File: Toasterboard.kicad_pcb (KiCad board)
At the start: 2 copper layers, 2 parts, among them U1 LM341T-05_TO220, U2 NE555P

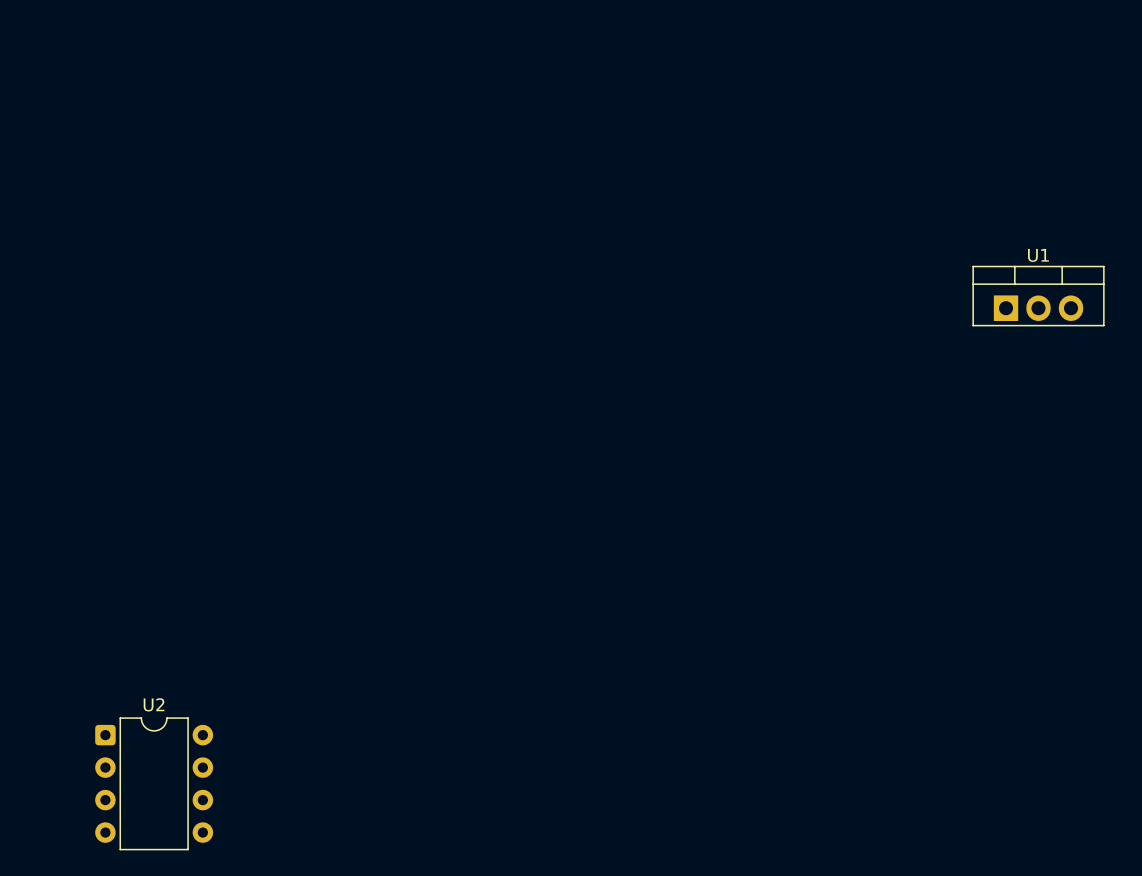
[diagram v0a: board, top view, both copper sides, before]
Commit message: feat: finished basic logics
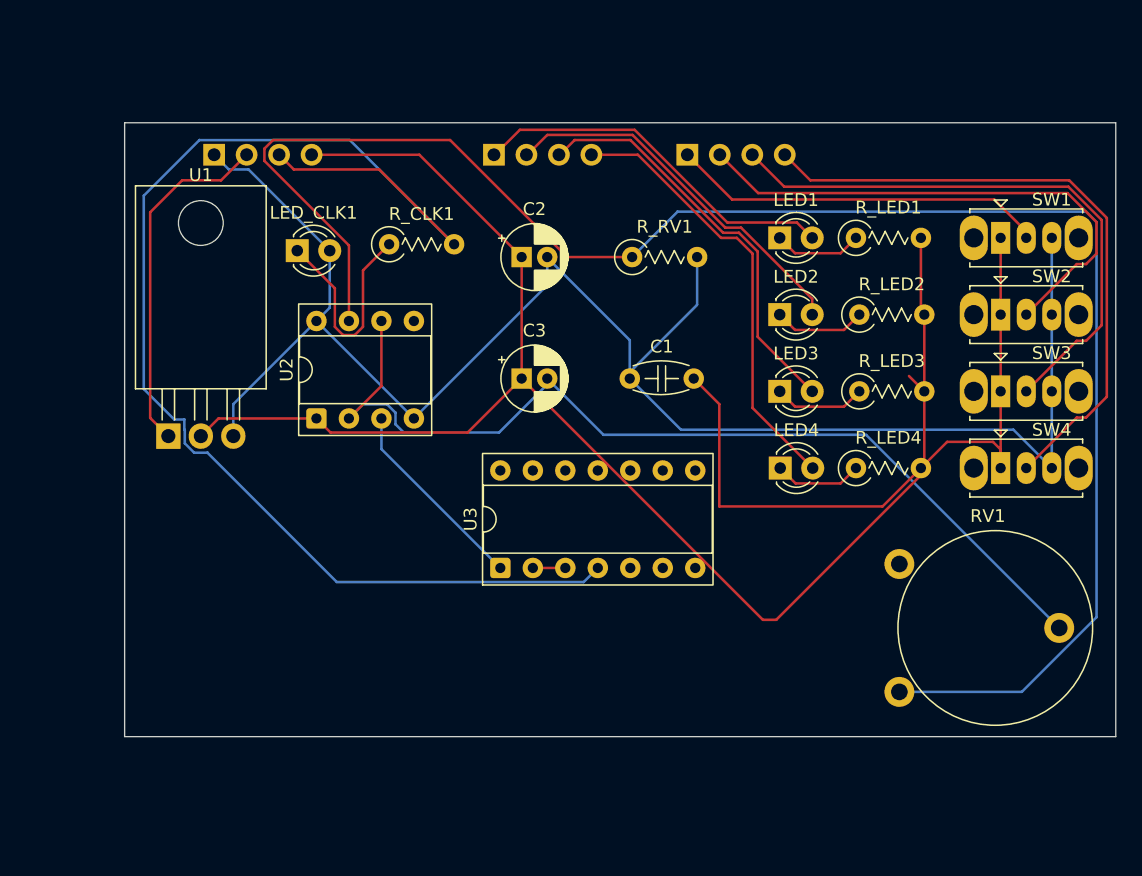
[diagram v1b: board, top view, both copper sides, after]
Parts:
- added C1: 0.01uF, PCM_Capacitor_THT_US_AKL:C_Disc_D5.0mm_W2.5mm_P5.00mm, F.Cu at (129.0, 88.5)
- added C2: 100uF, PCM_Capacitor_THT_US_AKL:CP_Radial_D5.0mm_P2.00mm, F.Cu at (120.5, 79.0)
- added C3: 100uF, PCM_Capacitor_THT_US_AKL:CP_Radial_D5.0mm_P2.00mm, F.Cu at (120.5, 88.5)
- added J1: Power, Connector_PinHeader_2.54mm:PinHeader_1x04_P2.54mm_Vertical, B.Cu at (96.5, 71.0)
- added J2: LEDs, Connector_PinHeader_2.54mm:PinHeader_1x04_P2.54mm_Vertical, B.Cu at (118.4, 71.0)
- added J3: Switches, Connector_PinHeader_2.54mm:PinHeader_1x04_P2.54mm_Vertical, B.Cu at (133.5, 71.0)
- added LED1: Red, LED_THT:LED_D3.0mm, F.Cu at (140.7, 77.5)
- added LED2: Red, LED_THT:LED_D3.0mm, F.Cu at (140.7, 83.5)
- added LED3: Red, LED_THT:LED_D3.0mm, F.Cu at (140.7, 89.5)
- added LED4: Red, LED_THT:LED_D3.0mm, F.Cu at (140.8, 95.5)
- added LED_CLK1: Green, LED_THT:LED_D3.0mm, F.Cu at (103.0, 78.5)
- added RV1: 10k, Potentiometer_THT:Potentiometer_Piher_PT-15-V02_Vertical, F.Cu at (150.1, 113.0)
- added R_CLK1: 1k, PCM_Resistor_THT_US_AKL:R_Axial_DIN0207_L6.3mm_D2.5mm_P5.08mm_Vertical, F.Cu at (110.2, 78.0)
- added R_LED1: 1k, PCM_Resistor_THT_US_AKL:R_Axial_DIN0207_L6.3mm_D2.5mm_P5.08mm_Vertical, F.Cu at (146.7, 77.5)
- added R_LED2: 1k, PCM_Resistor_THT_US_AKL:R_Axial_DIN0207_L6.3mm_D2.5mm_P5.08mm_Vertical, F.Cu at (146.9, 83.5)
- added R_LED3: 1k, PCM_Resistor_THT_US_AKL:R_Axial_DIN0207_L6.3mm_D2.5mm_P5.08mm_Vertical, F.Cu at (146.9, 89.5)
- added R_LED4: 1k, PCM_Resistor_THT_US_AKL:R_Axial_DIN0207_L6.3mm_D2.5mm_P5.08mm_Vertical, F.Cu at (146.7, 95.5)
- added R_RV1: 1k, PCM_Resistor_THT_US_AKL:R_Axial_DIN0207_L6.3mm_D2.5mm_P5.08mm_Vertical, F.Cu at (129.2, 79.0)
- added SW1: SW_SPDT, Button_Switch_THT:SW_Slide_SPDT_Straight_CK_OS102011MS2Q, F.Cu at (158.0, 77.5)
- added SW2: SW_SPDT, Button_Switch_THT:SW_Slide_SPDT_Straight_CK_OS102011MS2Q, F.Cu at (158.0, 83.5)
- added SW3: SW_SPDT, Button_Switch_THT:SW_Slide_SPDT_Straight_CK_OS102011MS2Q, F.Cu at (158.0, 89.5)
- added SW4: SW_SPDT, Button_Switch_THT:SW_Slide_SPDT_Straight_CK_OS102011MS2Q, F.Cu at (158.0, 95.5)
- added U3: 74LS14, Package_DIP:DIP-14_W7.62mm_Socket, F.Cu at (118.9, 103.3)
- U1: footprint Package_TO_SOT_THT:TO-220-3_Vertical -> Package_TO_SOT_THT:TO-220-3_Horizontal_TabDown
- U2: footprint Package_DIP:DIP-8_W7.62mm -> Package_DIP:DIP-8_W7.62mm_Socket
- moved U1 66.3 mm to (92.9, 93.0)
- moved U2 29.8 mm to (104.5, 91.6), turned to 90 degrees
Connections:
- U2 pad 2: unconnected-(U2-TRIG-Pad2) -> Net-(U2-THRES)
- U2 pad 4: unconnected-(U2-~{RST}-Pad4) -> +5V
- U2 pad 6: unconnected-(U2-THRES-Pad6) -> Net-(U2-THRES)
- U2 pad 7: unconnected-(U2-DISCH-Pad7) -> Net-(U2-DISCH)
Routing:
- net GND: track 0.00 -> 176.9 mm
- net Net-(U2-DISCH): track 0.00 -> 135.9 mm
- net +5V: track 0.00 -> 135.4 mm
- net /Clk: track 0.00 -> 104.4 mm
- net Net-(U2-THRES): track 0.00 -> 76.2 mm
- net Net-(J3-Pin_4): track 0.00 -> 49.8 mm
- net Net-(J3-Pin_3): track 0.00 -> 45.7 mm
- net Net-(J3-Pin_2): track 0.00 -> 41.6 mm
- net Net-(J2-Pin_4): track 0.00 -> 34.4 mm
- net Net-(J2-Pin_3): track 0.00 -> 32.2 mm
- net Net-(J3-Pin_1): track 0.00 -> 29.5 mm
- net Net-(J2-Pin_2): track 0.00 -> 29.5 mm
- net Net-(J2-Pin_1): track 0.00 -> 29.1 mm
- net +12V: track 0.00 -> 27.5 mm
- net Net-(LED_CLK1-K): track 0.00 -> 17.2 mm
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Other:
- board outline added: 77.5 x 48 mm

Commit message: feat: finish routing
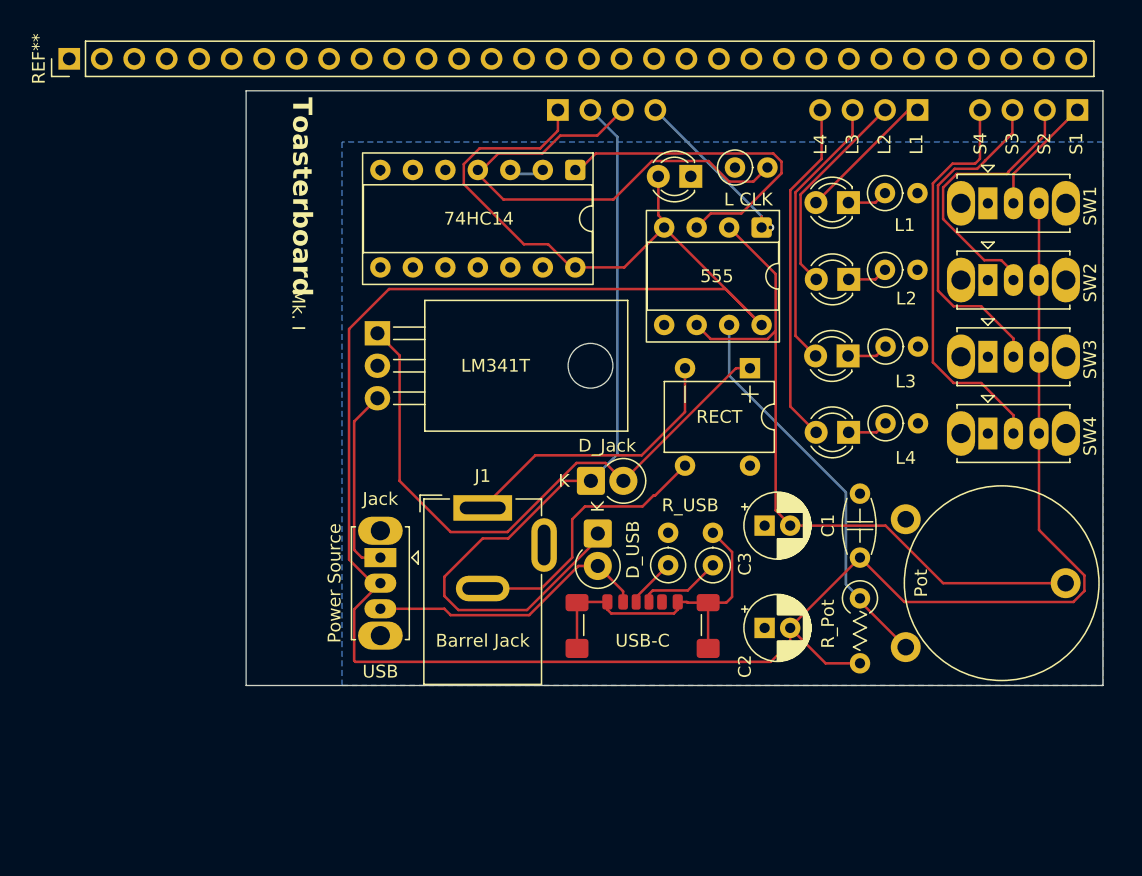
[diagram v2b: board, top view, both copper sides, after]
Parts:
- removed U1: LM341T-05_TO220, Package_TO_SOT_THT:TO-220-3_Horizontal_TabDown
- added D_Jack: 1N5817, Diode_THT:D_DO-41_SOD81_P2.54mm_Vertical_CathodeUp, F.Cu at (126.0, 96.5)
- added D_USB: 1N5817, Diode_THT:D_DO-41_SOD81_P2.54mm_Vertical_CathodeUp, F.Cu at (126.5, 100.6)
- added J1: Barrel Jack, Connector_BarrelJack:BarrelJack_GCT_DCJ200-10-A_Horizontal, F.Cu at (117.5, 98.6)
- added LM341T: LM341T-05_TO220, Package_TO_SOT_THT:TO-220-3_Horizontal_TabDown, F.Cu at (109.3, 85.0)
- added RECT: CS10D, PCM_Diode_THT_AKL:Diode_Bridge_DIP-4_W7.62mm_P5.08mm, F.Cu at (138.4, 87.7)
- added REF**: PinHeader_1x32_P2.54mm_Vertical, Connector_PinHeader_2.54mm:PinHeader_1x32_P2.54mm_Vertical, F.Cu at (85.2, 63.5)
- added R_USB1: 5.1k, PCM_Resistor_THT_US_AKL:R_Axial_DIN0207_L6.3mm_D2.5mm_P2.54mm_Vertical, F.Cu at (132.0, 103.1)
- added R_USB2: 5.1k, PCM_Resistor_THT_US_AKL:R_Axial_DIN0207_L6.3mm_D2.5mm_P2.54mm_Vertical, F.Cu at (135.5, 103.1)
- added SW_PWR1: SW_SPDT, Button_Switch_THT:SW_Slide_SPDT_Straight_CK_OS102011MS2Q, F.Cu at (109.5, 102.5)
- added USB-C: USB_C_Plug_USB2.0, Connector_USB:USB_C_Receptacle_GCT_USB4135-GF-A_6P_TopMnt_Horizontal, F.Cu at (130.0, 109.0)
- 74HC14: renamed from U3; value 74LS14 -> 74HC14
- L CLK: renamed from LED_CLK1
- R_CLK1, R_LED1, R_LED2, R_LED3, R_LED4: footprint PCM_Resistor_THT_US_AKL:R_Axial_DIN0207_L6.3mm_D2.5mm_P5.08mm_Vertical -> PCM_Resistor_THT_US_AKL:R_Axial_DIN0207_L6.3mm_D2.5mm_P2.54mm_Vertical
- moved 555 37.9 mm to (139.3, 76.7), turned to -90 degrees
- moved C2 34.7 mm to (139.5, 108.0)
- moved J3 33.3 mm to (151.5, 67.5), turned to 90 degrees
- moved R_Pot 32.1 mm to (147.0, 105.7), turned to -90 degrees
- moved 74HC14 31.7 mm to (124.7, 72.2), turned to -90 degrees
- moved L CLK 31.3 mm to (133.8, 72.7), turned to 180 degrees
- moved J4 30.7 mm to (164.0, 67.5), turned to 90 degrees
- moved R_CLK1 27.7 mm to (137.2, 72.0)
- moved J2 27.1 mm to (123.4, 67.5)
- moved C1 22.8 mm to (147.0, 102.5), turned to 90 degrees
- moved C3 22.2 mm to (139.5, 100.0)
- moved L2 6.06 mm to (146.1, 80.7), turned to 180 degrees
- moved L1 6.04 mm to (146.1, 74.7), turned to 180 degrees
- moved L4 6.03 mm to (146.1, 92.7), turned to 180 degrees
- moved L3 6.02 mm to (146.1, 86.7), turned to 180 degrees
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- renumbered U2 to 555, J1 to J2, J2 to J3, J3 to J4, LED1 to L1, LED2 to L2, LED3 to L3, LED4 to L4, R_RV1 to R_Pot
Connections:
- 74HC14 pad 14: (no net) -> +5V
- 74HC14 pad 7: (no net) -> GND
- J2 pad 2: +12V -> +VDC
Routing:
- net GND: track 176.9 -> 40.1 mm, vias 0 -> 17
- net Net-(U2-DISCH): track 135.9 -> 30.9 mm
- net +5V: track 135.4 -> 210.5 mm
- net /Clk: track 104.4 -> 39.3 mm
- net +VDC: track 0.00 -> 62.0 mm
- net Net-(D_JACK1-A): track 0.00 -> 47.8 mm
- net +12V: track 27.5 -> 0.00 mm
- net Net-(D_USB1-A): track 0.00 -> 22.4 mm
- net Net-(D_RECT1-1): track 0.00 -> 22.4 mm
- net Net-(D_RECT1--): track 0.00 -> 21.6 mm
- net Net-(U2-THRES): track 76.2 -> 55.6 mm
- net Net-(J4-Pin_1): track 29.5 -> 9.37 mm
- net Net-(J4-Pin_2): track 41.6 -> 22.0 mm
- net Net-(J4-Pin_3): track 45.7 -> 26.5 mm
- net Net-(J3-Pin_1): track 29.1 -> 10.9 mm
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- added copper zone on B.Cu, net GND
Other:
- board size 77.5 x 48 mm -> 67 x 46.5 mm
- board text added: "Jack"
- board text added: "L1"
- board text added: "L2"
- board text added: "L3"
- board text added: "L4"
- board text added: "Mk. I"
- board text added: "Power Source"
- board text added: "R_USB"
- board text added: "S1"
- board text added: "S2"
- board text added: "S3"
- board text added: "S4"
- board text added: "SW2"
- board text added: "Toasterboard"
- board text added: "USB"
